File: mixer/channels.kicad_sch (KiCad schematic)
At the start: 21 parts, among them J8 AVR-ISP-6, Q1 NMOS, U2 TL074, U3 DG403, U4 TL074, U5 TL072, U6 ATtiny24-20SS, U7 TL074

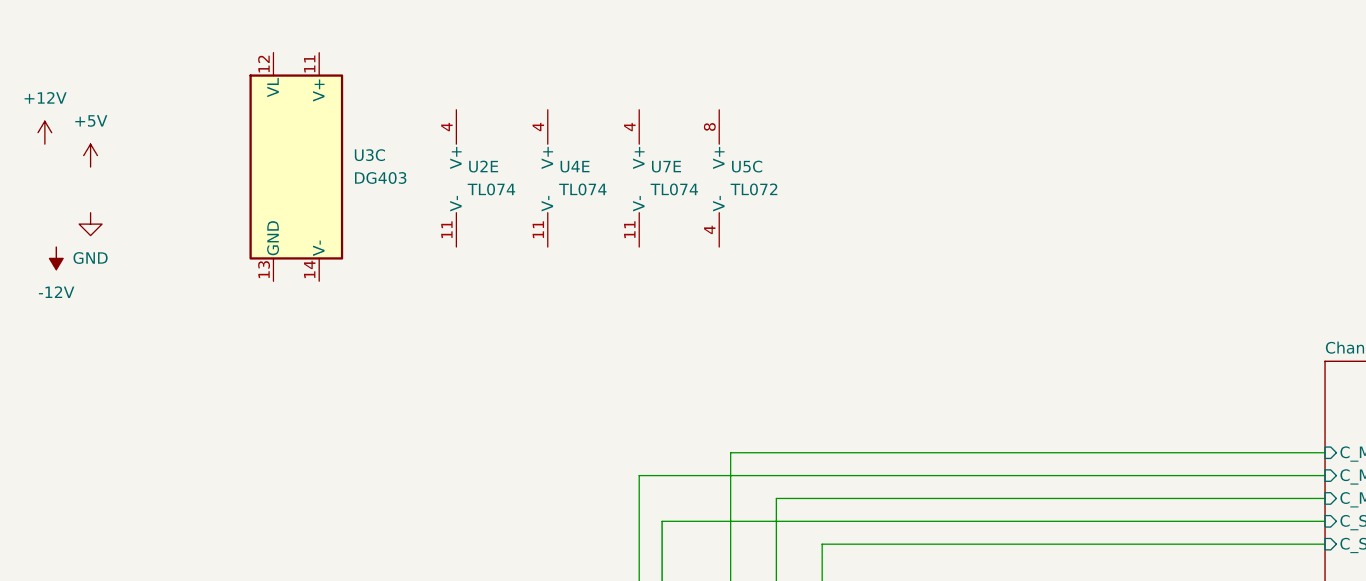
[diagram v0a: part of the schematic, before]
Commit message: making progress on the outline
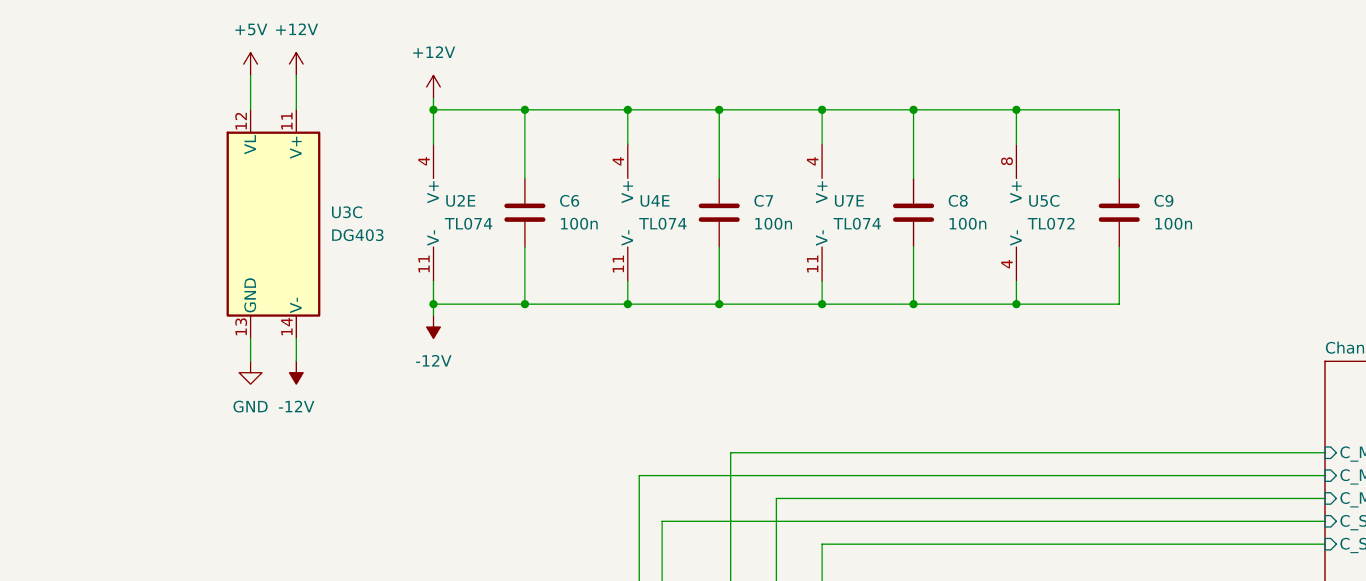
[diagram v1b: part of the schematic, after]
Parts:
- added C6, C7, C8, C9: 100n, Capacitor_SMD:C_0603_1608Metric, symbol Device:C
- C5: footprint (none) -> Capacitor_SMD:C_0603_1608Metric
- J8: footprint (none) -> _project:IVR_PADS
- R13, R14, R15, R16, R17, R18, R19, R20, R21, R22, R23, R24: footprint (none) -> Resistor_SMD:R_0603_1608Metric
- U2, U4, U7: footprint (none) -> Package_SO:SOIC-14_3.9x8.7mm_P1.27mm
- U5: footprint (none) -> Package_SO:SOIC-8_3.9x4.9mm_P1.27mm
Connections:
- net +12V: now also U2.4 (V+), U3.11 (V+), U4.4 (V+), U5.8 (V+), U7.4 (V+), C6.1, C7.1, C8.1, C9.1
- net +5V: now also U3.12 (VL)
- net -12V: now also U2.11 (V-), U3.14 (V-), U4.11 (V-), U5.4 (V-), U7.11 (V-), C6.2, C7.2, C8.2, C9.2
- net GND: now also U3.13 (GND)
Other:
- moved on the sheet: U2E, U3C, U4E, U5C, U7E
